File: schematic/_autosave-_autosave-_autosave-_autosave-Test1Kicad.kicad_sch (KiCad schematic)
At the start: 73 parts, among them IC1 BMI055, J1 Power Module 1, J10 CAP & ADC IN, J11 SPI Port, J12 I2C A, J13 FMU PWM OUT, J14 PPM RC, J15 2908-05WB-MG, J16 RC, J17 SBUS, J18 IO/PWM out, J2 Power Module 2, J3 USB, J4 Telemetry 1, J5 Telemetry 2, J6 UART & I2C B, J7 CAN 1, J8 CAN 2, J9 GPS Module, U1 STM32F765IIKx, U10 TJA1051TK-3, U11 LT3080xDD, U12 LP5907MFX-3.3, U3 IST8310, U4 ICM-20602, U5 ICM-20689, U6 MS5611-01BA, U8 STM32F103V8Tx, U9 TJA1051TK-3, Y1 ABM2-8.000MHZ-D4Y-T

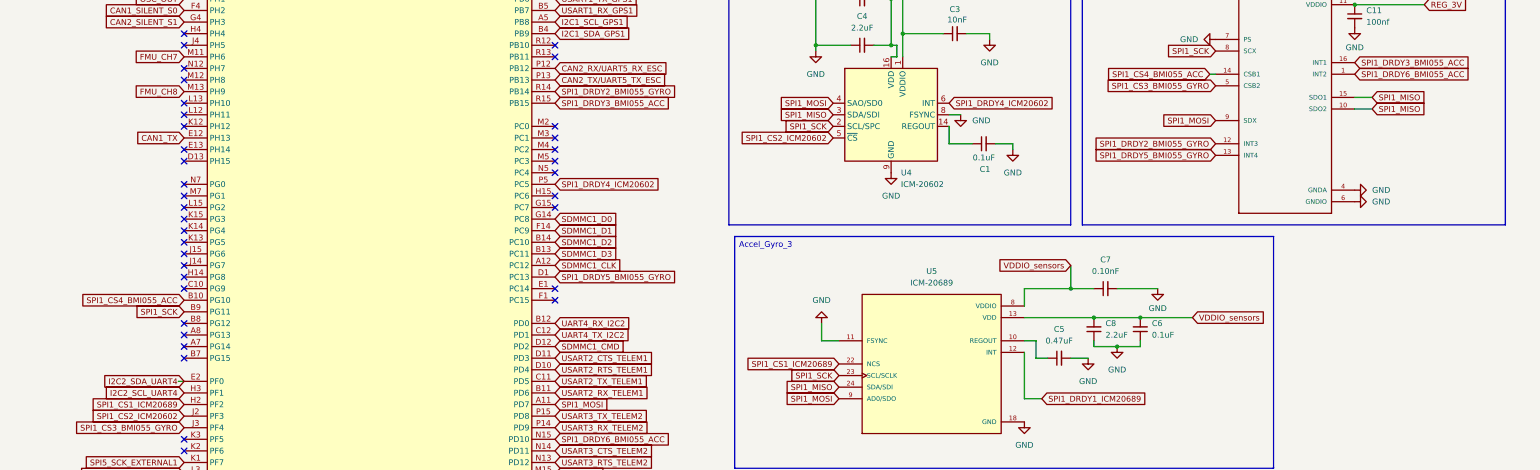
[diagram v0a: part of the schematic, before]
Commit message: EVEN MORE ERRORS!!
only a few to go can see the end
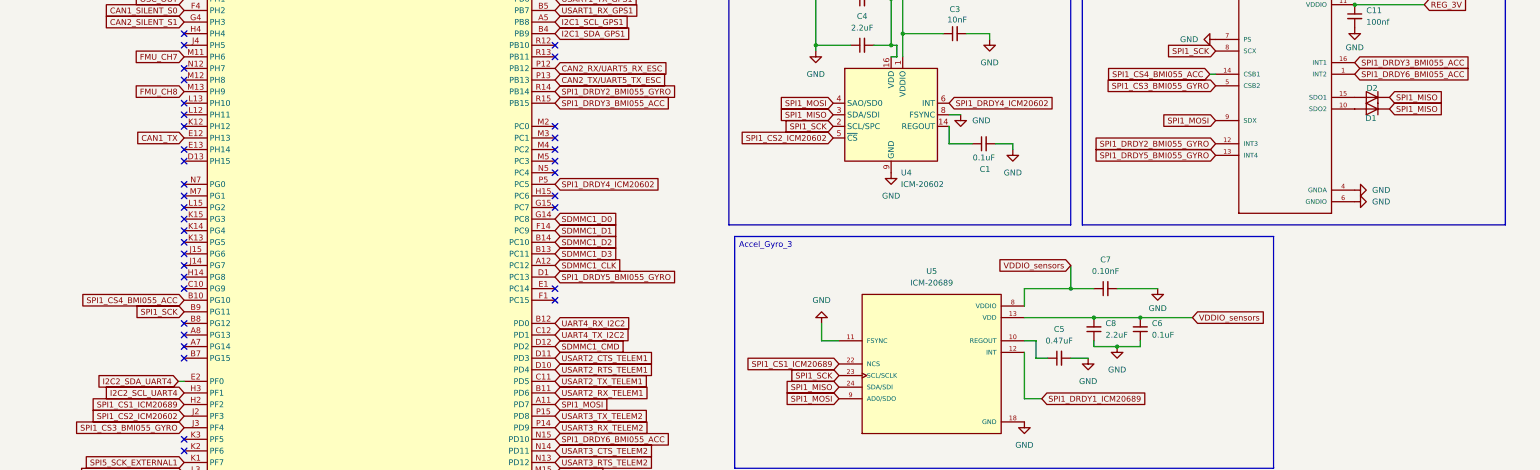
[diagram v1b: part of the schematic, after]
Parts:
- added D1, D2: 1N4148WT, Diode_SMD:D_SOD-523, symbol Diode:1N4148WT
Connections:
- net SPI1_MISO: now also D1.1 (K), D2.1 (K); no longer IC1.10 (SDO2), IC1.15 (SDO1)
- new net: D2.2 (A), IC1.15 (SDO1)
- new net: D1.2 (A), IC1.10 (SDO2)
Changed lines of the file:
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@@
 	(wire
 		(pts
-			(xy 384.81 116.84) (xy 381 116.84)
-		)
-		(stroke
-			(width 0)
-			(type default)
-		)
-	)
-	(wire
-		(pts
 			(xy 289.56 74.93) (xy 289.56 73.66)
 		)
@@
 	(wire
 		(pts
+			(xy 123.19 179.07) (xy 124.46 179.07)
+		)
+		(stroke
+			(width 0)
+			(type default)
+		)
+	)
+	(wire
+		(pts
 			(xy 308.61 158.75) (xy 308.61 162.56)
 		)
@@
 	(wire
 		(pts
-			(xy 123.19 179.07) (xy 124.46 179.07)
-		)
-		(stroke
-			(width 0)
-			(type default)
-		)
-	)
-	(wire
-		(pts
 			(xy 318.77 158.75) (xy 323.85 158.75)
 		)
@@
 	(wire
 		(pts
-			(xy 381 119.38) (xy 384.81 119.38)
-		)
-		(stroke
-			(width 0)
-			(type default)
-		)
-	)
-	(wire
-		(pts
 			(xy 523.24 38.1) (xy 525.78 38.1)
 		)
@@
 	(global_label "I2C2_SDA_UART4"
 		(shape input)
-		(at 124.46 179.07 180)
+		(at 123.19 179.07 180)
 		(fields_autoplaced yes)
 		(effects
@@
 		)
 		(property "Intersheetrefs" "${INTERSHEET_REFS}"
-			(at 105.8115 179.07 0)
+			(at 104.5415 179.07 0)
 			(effects
 				(font
@@
 		)
 	)
+	(global_label "SPI1_MISO"
+		(shape input)
+		(at 388.62 116.84 0)
+		(fields_autoplaced yes)
+		(effects
+			(font
+				(size 1.27 1.27)
+			)
+			(justify left)
+		)
+		(property "Intersheetrefs" "${INTERSHEET_REFS}"
+			(at 401.4628 116.84 0)
+			(effects
+				(font
+					(size 1.27 1.27)
+				)
+				(justify left)
+				(hide yes)
+			)
+		)
+	)
 	(global_label "I2C4_SCL_EXTERNAL2"
 		(shape input)
@@
 		)
 	)
+	(global_label "SPI1_MISO"
+		(shape input)
+		(at 388.62 119.38 0)
+		(fields_autoplaced yes)
+		(effects
+			(font
+				(size 1.27 1.27)
+			)
+			(justify left)
+		)
+		(property "Intersheetrefs" "${INTERSHEET_REFS}"
+			(at 401.4628 119.38 0)
+			(effects
+				(font
+					(size 1.27 1.27)
+				)
+				(justify left)
+				(hide yes)
+			)
+		)
+	)
 	(global_label "UART4_RX_I2C2"
 		(shape input)
@@
 		)
 	)
-	(global_label "SPI1_MISO"
-		(shape input)
-		(at 384.81 119.38 0)
-		(fields_autoplaced yes)
-		(effects
-			(font
-				(size 1.27 1.27)
-			)
-			(justify left)
-		)
-		(property "Intersheetrefs" "${INTERSHEET_REFS}"
-			(at 397.6528 119.38 0)
-			(effects
-				(font
-					(size 1.27 1.27)
-				)
-				(justify left)
-				(hide yes)
-			)
-		)
-	)
 	(global_label "USART3_CTS_TELEM2"
 		(shape input)
@@
 		)
 	)
-	(global_label "SPI1_MISO"
-		(shape input)
-		(at 384.81 116.84 0)
-		(fields_autoplaced yes)
-		(effects
-			(font
-				(size 1.27 1.27)
-			)
-			(justify left)
-		)
-		(property "Intersheetrefs" "${INTERSHEET_REFS}"
-			(at 397.6528 116.84 0)
-			(effects
-				(font
-					(size 1.27 1.27)
-				)
-				(justify left)
-				(hide yes)
-			)
-		)
-	)
 	(global_label "TIM1_CH1"
 		(shape input)
@@
 	)
 	(symbol
+		(lib_id "Diode:1N4148WT")
+		(at 384.81 116.84 180)
+		(unit 1)
+		(exclude_from_sim no)
+		(in_bom yes)
+		(on_board yes)
+		(dnp no)
+		(property "Reference" "D2"
+			(at 384.81 114.808 0)
+			(effects
+				(font
+					(size 1.27 1.27)
+				)
+			)
+		)
+		(property "Value" "1N4148WT"
+			(at 384.81 112.268 0)
+			(effects
+				(font
+					(size 1.27 1.27)
+				)
+				(hide yes)
+			)
+		)
+		(property "Footprint" "Diode_SMD:D_SOD-523"
+			(at 384.81 112.395 0)
+			(effects
+				(font
+					(size 1.27 1.27)
+				)
+				(hide yes)
+			)
+		)
+		(property "Datasheet" "https://www.diodes.com/assets/Datasheets/ds30396.pdf"
+			(at 384.81 116.84 0)
+			(effects
+				(font
+					(size 1.27 1.27)
+				)
+				(hide yes)
+			)
+		)
+		(property "Description" "75V 0.15A Fast switching Diode, SOD-523"
+			(at 384.81 116.84 0)
+			(effects
+				(font
+					(size 1.27 1.27)
+				)
+				(hide yes)
+			)
+		)
+		(property "Sim.Device" "D"
+			(at 384.81 116.84 0)
+			(effects
+				(font
+					(size 1.27 1.27)
+				)
+				(hide yes)
+			)
+		)
+		(property "Sim.Pins" "1=K 2=A"
+			(at 384.81 116.84 0)
+			(effects
+				(font
+					(size 1.27 1.27)
+				)
+				(hide yes)
+			)
+		)
+		(pin "1"
+		)
+		(pin "2"
+		)
+		(instances
+			(project "_autosave-_autosave-_autosave-_autosave-Test1Kicad"
+				(path "/8ed38441-7d4e-4e89-870f-07e11c6dce38"
+					(reference "D2")
+					(unit 1)
+				)
+			)
+		)
+	)
+	(symbol
 		(lib_id "power:GND")
 		(at 513.08 210.82 90)
@@
 					(unit 1)
 				)
+			)
+		)
+	)
+	(symbol
+		(lib_id "Diode:1N4148WT")
+		(at 384.81 119.38 180)
+		(unit 1)
+		(exclude_from_sim no)
+		(in_bom yes)
+		(on_board yes)
+		(dnp no)
+		(property "Reference" "D1"
+			(at 384.556 121.412 0)
+			(effects
+				(font
+					(size 1.27 1.27)
+				)
+			)
+		)
+		(property "Value" "1N4148WT"
+			(at 384.81 114.808 0)
+			(effects
+				(font
+					(size 1.27 1.27)
+				)
+				(hide yes)
+			)
+		)
+		(property "Footprint" "Diode_SMD:D_SOD-523"
+			(at 384.81 114.935 0)
+			(effects
+				(font
+					(size 1.27 1.27)
+				)
+				(hide yes)
+			)
+		)
+		(property "Datasheet" "https://www.diodes.com/assets/Datasheets/ds30396.pdf"
+			(at 384.81 119.38 0)
+			(effects
+				(font
+					(size 1.27 1.27)
+				)
+				(hide yes)
+			)
+		)
+		(property "Description" "75V 0.15A Fast switching Diode, SOD-523"
+			(at 384.81 119.38 0)
+			(effects
+				(font
+					(size 1.27 1.27)
+				)
+				(hide yes)
+			)
+		)
+		(property "Sim.Device" "D"
+			(at 384.81 119.38 0)
+			(effects
+				(font
+					(size 1.27 1.27)
+				)
+				(hide yes)
+			)
+		)
+		(property "Sim.Pins" "1=K 2=A"
+			(at 384.81 119.38 0)
+			(effects
+				(font
+					(size 1.27 1.27)
+				)
+				(hide yes)
+			)
+		)
+		(pin "1"
+		)
+		(pin "2"
+		)
+		(instances
+			(project ""
+				(path "/8ed38441-7d4e-4e89-870f-07e11c6dce38"
+					(reference "D1")
+					(unit 1)
+				)
